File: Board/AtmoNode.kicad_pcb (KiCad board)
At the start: 4 copper layers, 46 x 35 mm, 67 parts, among them J1 USB_B_Micro, J2 OLED_I2C, Q1 S9012, Q2 S9012, SW2 USER, SW3 FLASH, U1 AP1117-33, U2 CH340C, U3 ESP8266EX, U4 W25Q16JVSSIQ, U5 BME280, Y1 26MHz

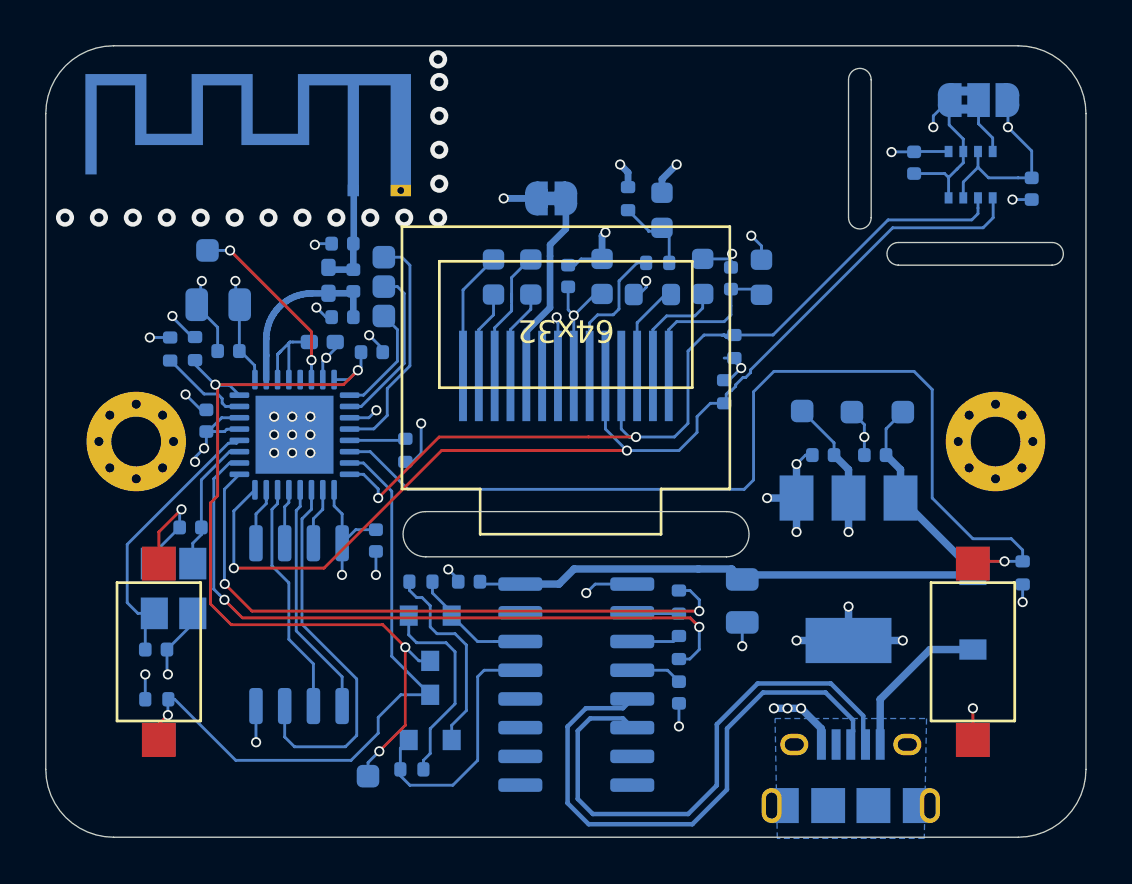
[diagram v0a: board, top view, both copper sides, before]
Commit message: df:
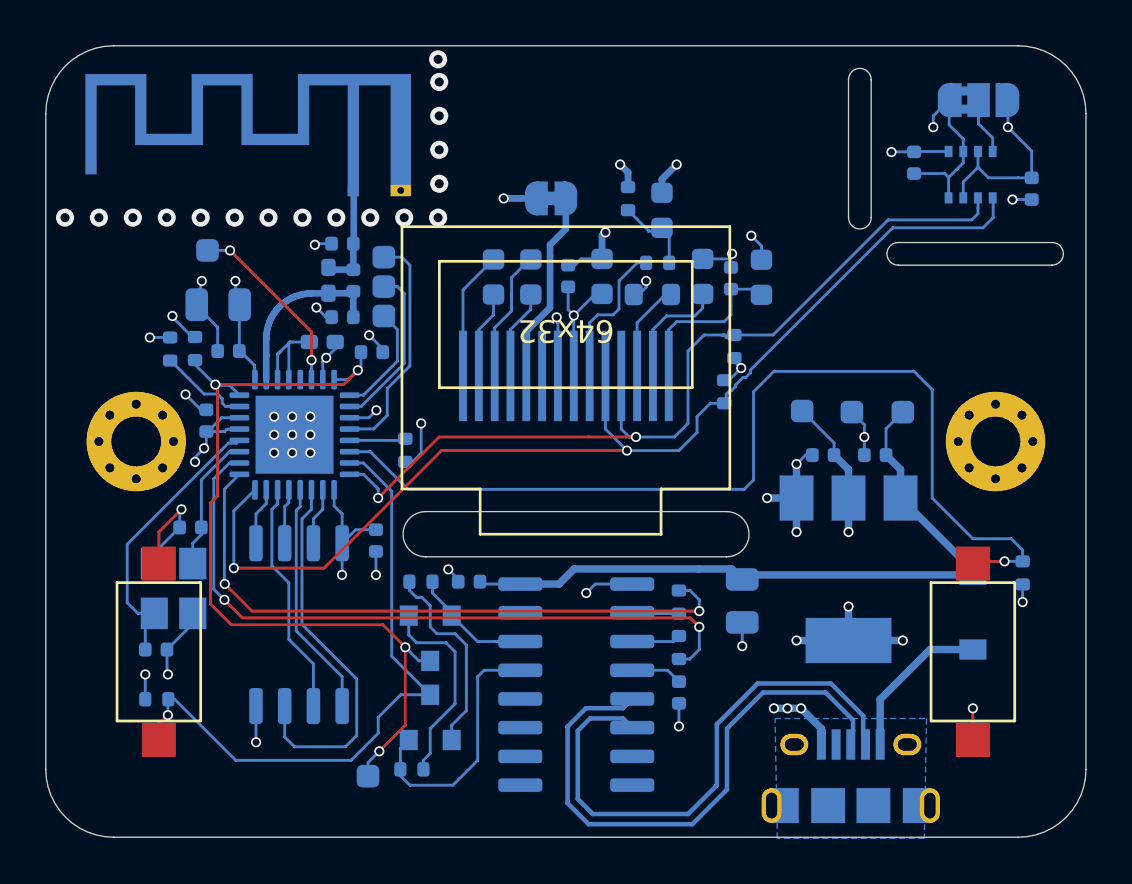
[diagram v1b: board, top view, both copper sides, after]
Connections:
- J1 pad 4: Net-(J1-Pad4) -> unconnected-(J1-Pad4)
- J1 pad 6: Net-(J1-Pad6) -> unconnected-(J1-Pad6)
- J2 pad 6: Net-(J2-Pad6) -> unconnected-(J2-Pad6)
- U2 pad 10: Net-(U2-Pad10) -> unconnected-(U2-Pad10)
- U2 pad 11: Net-(U2-Pad11) -> unconnected-(U2-Pad11)
- U2 pad 12: Net-(U2-Pad12) -> unconnected-(U2-Pad12)
- U2 pad 15: Net-(U2-Pad15) -> unconnected-(U2-Pad15)
- U2 pad 7: Net-(U2-Pad7) -> unconnected-(U2-Pad7)
- U2 pad 8: Net-(U2-Pad8) -> unconnected-(U2-Pad8)
- U2 pad 9: Net-(U2-Pad9) -> unconnected-(U2-Pad9)
- U3 pad 5: Net-(U3-Pad5) -> unconnected-(U3-Pad5)
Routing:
- added copper zone on B.Cu, net unconnected-(J1-Pad6)
- removed copper zone on B.Cu, net Net-(J1-Pad6)
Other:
- net class Default removed
- net class POWER removed
- net class RF 50Ohm removed
- board text added: "~{RST}"
- board text removed: "~RST"
